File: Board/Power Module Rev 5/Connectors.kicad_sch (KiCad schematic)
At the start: 4 parts, among them J1 9-6437287-8, J3 Conn_01x16_Pin

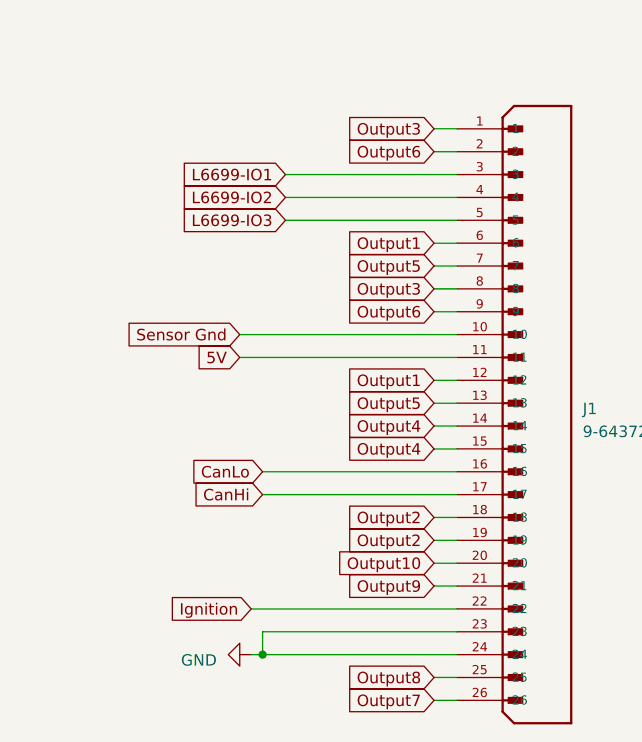
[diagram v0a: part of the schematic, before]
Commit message: Board Progress
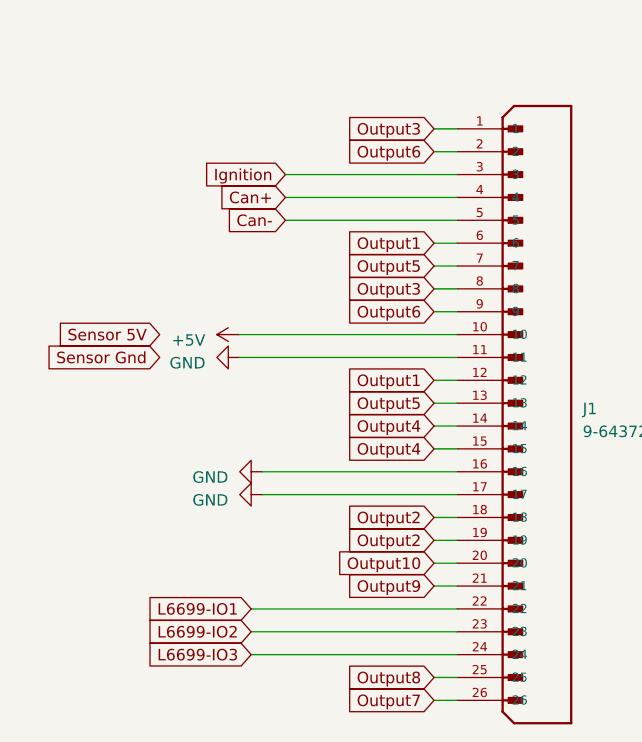
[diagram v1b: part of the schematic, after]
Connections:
- net 5V is gone; now on net GND: J1.11
- net CanHi is gone; now on net GND: J1.17
- net CanLo is gone; now on net GND: J1.16
- net GND: no longer J1.23, J1.24
- net Ignition: now also J1.3; no longer J1.22
- net L6699-IO1: now also J1.22; no longer J1.3
- net L6699-IO2: now also J1.23; no longer J1.4
- net L6699-IO3: now also J1.24; no longer J1.5
- net Sensor Gnd: no longer J1.10
- new net +5V: J1.10
- new net Can+: J1.4
- new net Can-: J1.5

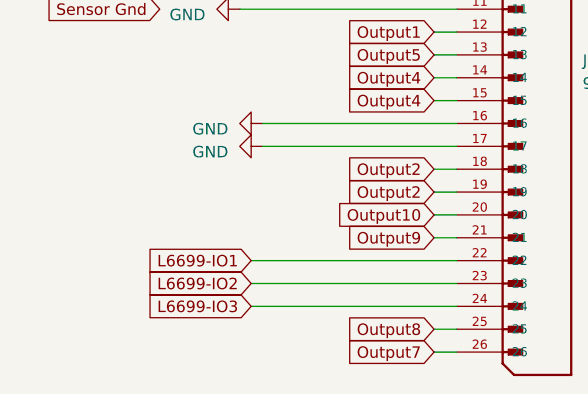
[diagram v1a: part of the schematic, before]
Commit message: Update Board
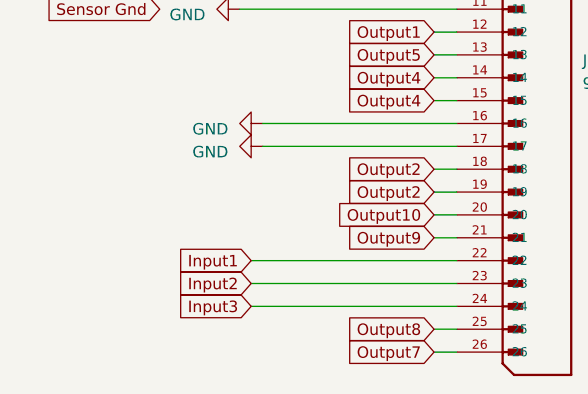
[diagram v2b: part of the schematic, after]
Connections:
- net L6699-IO1 renamed Input1
- net L6699-IO2 renamed Input2
- net L6699-IO3 renamed Input3
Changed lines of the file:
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@@
     )
   )
-  (global_label "L6699-IO2" (shape input) (at 60.96 105.41 180) (fields_autoplaced)
+  (global_label "Input2" (shape input) (at 60.96 105.41 180) (fields_autoplaced)
     (effects (font (size 1.27 1.27)) (justify right))
-    (property "Intersheetrefs" "${INTERSHEET_REFS}" (at 47.4709 105.41 0)
+    (property "Intersheetrefs" "${INTERSHEET_REFS}" (at 52.0672 105.41 0)
       (effects (font (size 1.27 1.27)) (justify right) hide)
     )
@@
     )
   )
-  (global_label "L6699-IO3" (shape input) (at 60.96 107.95 180) (fields_autoplaced)
+  (global_label "Input3" (shape input) (at 60.96 107.95 180) (fields_autoplaced)
     (effects (font (size 1.27 1.27)) (justify right))
-    (property "Intersheetrefs" "${INTERSHEET_REFS}" (at 47.4709 107.95 0)
+    (property "Intersheetrefs" "${INTERSHEET_REFS}" (at 52.0672 107.95 0)
       (effects (font (size 1.27 1.27)) (justify right) hide)
     )
@@
     )
   )
-  (global_label "L6699-IO1" (shape input) (at 60.96 102.87 180) (fields_autoplaced)
+  (global_label "Input1" (shape input) (at 60.96 102.87 180) (fields_autoplaced)
     (effects (font (size 1.27 1.27)) (justify right))
-    (property "Intersheetrefs" "${INTERSHEET_REFS}" (at 47.4709 102.87 0)
+    (property "Intersheetrefs" "${INTERSHEET_REFS}" (at 52.0672 102.87 0)
       (effects (font (size 1.27 1.27)) (justify right) hide)
     )

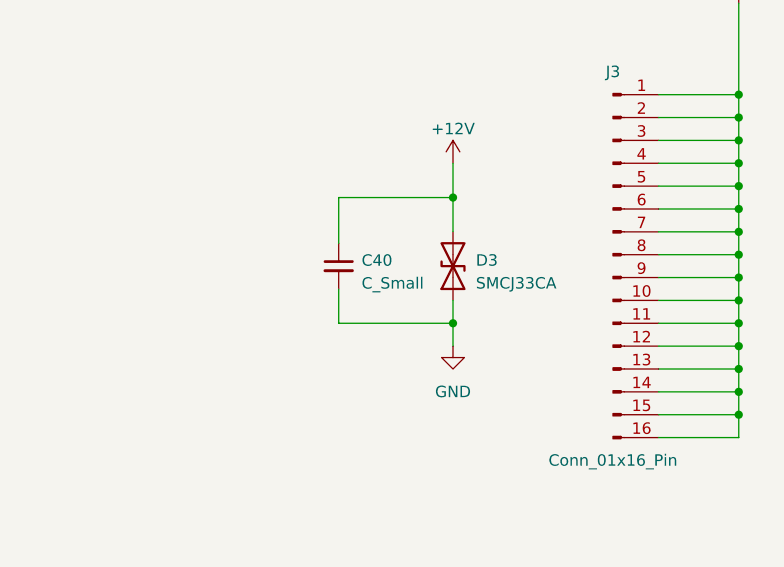
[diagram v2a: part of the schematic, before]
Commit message: Update Board
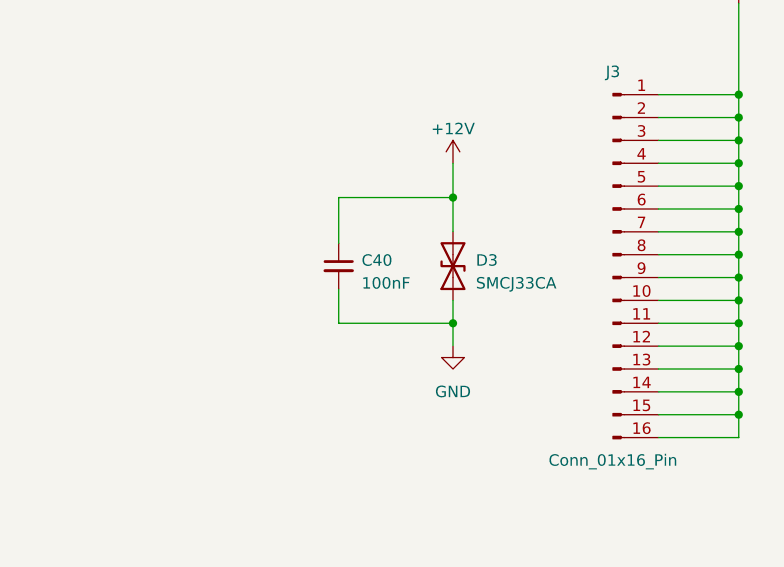
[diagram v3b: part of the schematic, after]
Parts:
- C40: value C_Small -> 100nF; footprint (none) -> Capacitor_SMD:C_0603_1608Metric_Pad1.08x0.95mm_HandSolder
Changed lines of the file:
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@@
       (effects (font (size 1.27 1.27)) (justify left))
     )
-    (property "Value" "C_Small" (at 233.68 52.7113 0)
+    (property "Value" "100nF" (at 233.68 52.7113 0)
       (effects (font (size 1.27 1.27)) (justify left))
     )
-    (property "Footprint" "" (at 231.14 50.8 0)
+    (property "Footprint" "Capacitor_SMD:C_0603_1608Metric_Pad1.08x0.95mm_HandSolder" (at 231.14 50.8 0)
       (effects (font (size 1.27 1.27)) hide)
     )
